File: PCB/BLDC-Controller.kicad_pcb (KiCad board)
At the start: 2 copper layers, 73 parts, among them Q1 Q_NMOS_GDS, Q2 Q_NMOS_GDS, Q3 Q_NMOS_GDS, Q4 Q_NMOS_GDS, Q5 Q_NMOS_GDS, Q6 Q_NMOS_GDS, U1 UCC27282DRM, U2 UCC27282DRM, U3 UCC27282DRM, U4 STM32F051K6Ux, U5 INA180A3, U6 TPS62933, Y1 8M

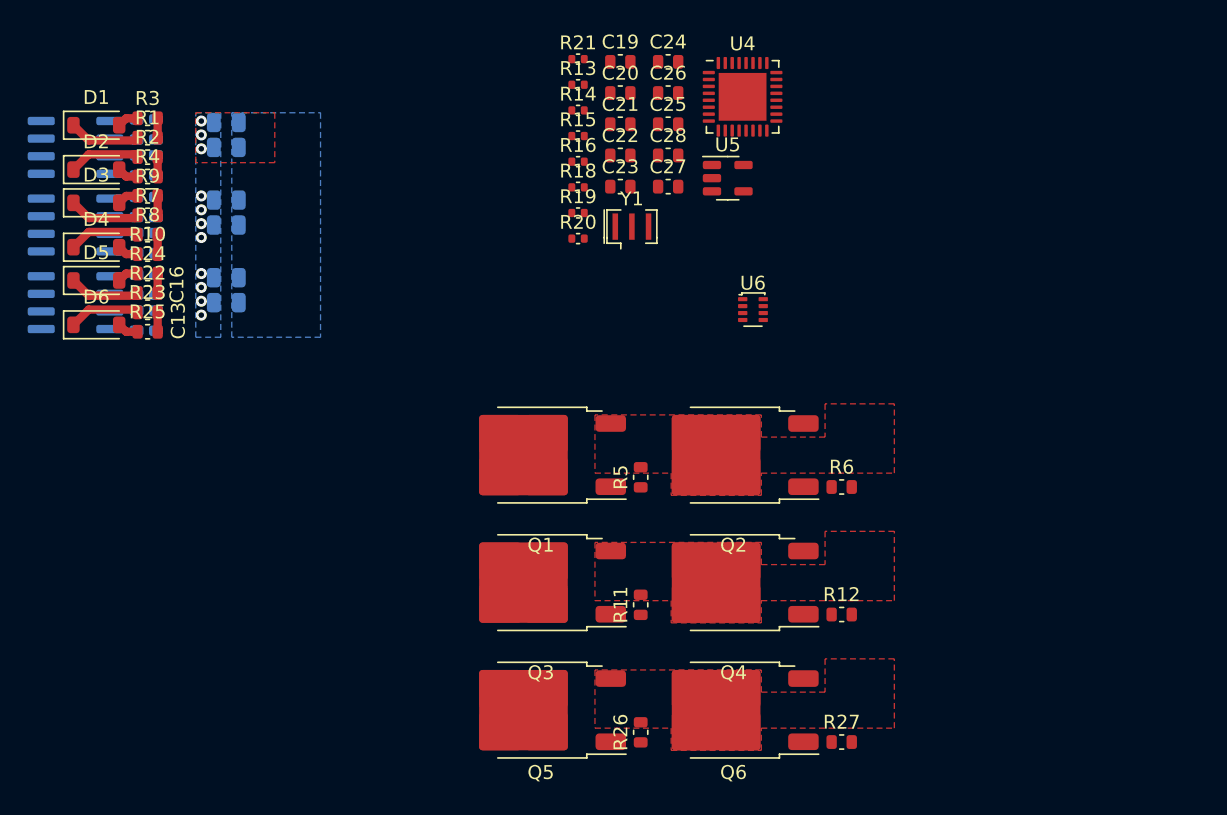
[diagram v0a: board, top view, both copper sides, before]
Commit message: f
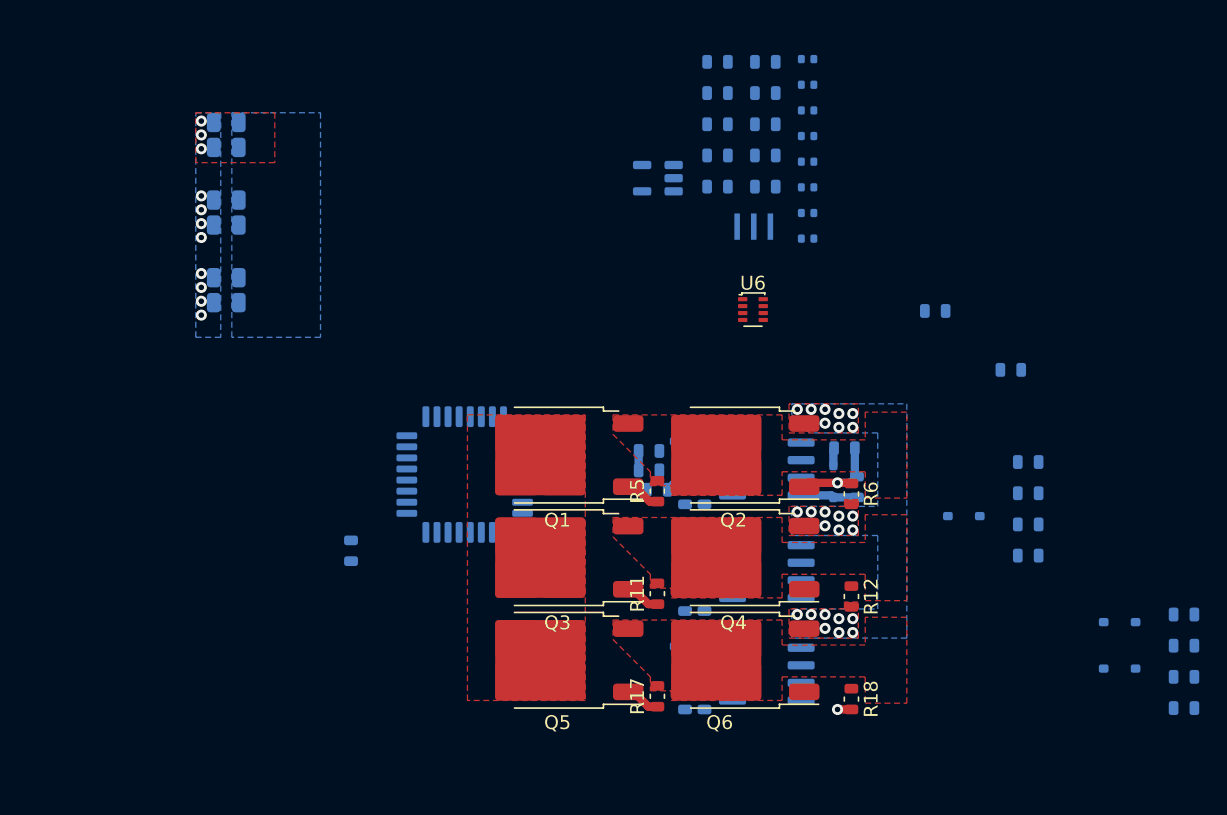
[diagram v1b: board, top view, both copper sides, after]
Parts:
- removed the C15 at (115.7, 95.4)
- removed the C3 at (115.7, 84.2)
- removed the C9 at (115.7, 89.8)
- removed the R22 at (116.5, 93.4)
- removed R23: 22, Ariamelon-Device:R_0603_1608Metric
- removed the R24 at (116.5, 92.0)
- removed the R25 at (116.5, 96.2)
- added L1: L_Small, Ariamelon-Device:L_0603_1608Metric, B.Cu at (153.3, 107.6)
- added L2: L_Small, Ariamelon-Device:L_0603_1608Metric, B.Cu at (178.8, 99.0)
- added L3: L_Small, Ariamelon-Device:L_0603_1608Metric, B.Cu at (173.3, 94.7)
- added R13: 10, Ariamelon-Device:R_0603_1608Metric, B.Cu at (180.1, 105.6)
- added R14: 10, Ariamelon-Device:R_0603_1608Metric, B.Cu at (180.1, 107.8)
- added R15: 22, Ariamelon-Device:R_0603_1608Metric, B.Cu at (180.1, 110.1)
- added R16: 22, Ariamelon-Device:R_0603_1608Metric, B.Cu at (180.1, 112.3)
- C16: renamed from C19; moved to B.Cu
- C17: renamed from C20; moved to B.Cu
- C18: renamed from C21; moved to B.Cu
- C19: renamed from C22; moved to B.Cu
- C20: renamed from C23; moved to B.Cu
- C21: renamed from C24; moved to B.Cu
- C22: renamed from C26; moved to B.Cu
- C23: renamed from C25; moved to B.Cu
- C24: renamed from C28; moved to B.Cu
- C25: renamed from C27; moved to B.Cu
- D1, D2, D3, D4, D5, D6: footprint Diode_SMD:D_SOD-123 -> Ariamelon-Device:D_SOD-323; moved to B.Cu
- Q1, Q2, Q3, Q4, Q5, Q6: footprint Package_TO_SOT_SMD:TO-252-2 -> Ariamelon-Package:TO-252-2
- R1, R2, R7, R8: value 22 -> 10; moved to B.Cu
- R10, R3, R4, R9: value 10 -> 22; moved to B.Cu
- R19: renamed from R21; moved to B.Cu
- R20: renamed from R13; moved to B.Cu
- R21: renamed from R14; moved to B.Cu
- R22: renamed from R15; moved to B.Cu
- R24: renamed from R16; moved to B.Cu
- R25: renamed from R18; moved to B.Cu
- R26: renamed from R19; moved to B.Cu
- R27: renamed from R20; moved to B.Cu
- U1, U2, U3: value UCC27282DRM -> UCC27211ADRM
- U4: value STM32F051K6Ux -> STM32F051K6Tx; footprint Package_DFN_QFN:QFN-32-1EP_5x5mm_P0.5mm_EP3.45x3.45mm -> Package_QFP:LQFP-32_7x7mm_P0.8mm; moved to B.Cu
- U5, Y1: moved to B.Cu
- moved R9 82.4 mm to (191.3, 121.1), turned to 180 degrees
- moved R10 81.6 mm to (191.3, 123.3), turned to 180 degrees
- moved R8 80.4 mm to (191.3, 118.8), turned to 180 degrees
- moved R7 80.1 mm to (191.3, 116.6), turned to 180 degrees
- moved D4 79.8 mm to (186.7, 120.5), turned to 180 degrees
- moved D3 79.8 mm to (186.7, 117.2), turned to 180 degrees
- moved D6 64.1 mm to (175.4, 109.5), turned to 180 degrees
- moved D2 57.7 mm to (166.0, 107.0), turned to 90 degrees
- moved U3 56.6 mm to (161.2, 120.9), turned to 0 degrees
- moved R4 55.9 mm to (167.7, 107.4), turned to 90 degrees
- moved U2 55.8 mm to (161.2, 113.5), turned to 0 degrees
- moved U1 55.0 mm to (161.2, 106.1), turned to 0 degrees
- moved R2 54.5 mm to (166.8, 104.6)
- moved C12 50.7 mm to (156.7, 122.7)
- moved D5 50.4 mm to (155.7, 118.9), turned to 180 degrees
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- renumbered C12 to C10, C13 to C11, C14 to C12, C16 to C13, C17 to C14, C18 to C15, C4 to C3, C5 to C4, C6 to C5, C7 to C6, C8 to C7, C10 to C8, C11 to C9, R26 to R17, R27 to R18
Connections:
- R1 pad 1: Net-(D1-K) -> Net-(D1-A)
- R10 pad 1: Net-(D4-A) -> Net-(D4-K)
- R2 pad 1: Net-(D2-K) -> Net-(D2-A)
- R3 pad 1: Net-(D1-A) -> Net-(D1-K)
- R4 pad 1: Net-(D2-A) -> Net-(D2-K)
- R7 pad 1: Net-(D3-K) -> Net-(D3-A)
- R8 pad 1: Net-(D4-K) -> Net-(D4-A)
- R9 pad 1: Net-(D3-A) -> Net-(D3-K)
- U4 pad 13: /MCU/LI_C -> /MCU/LI_A
- U4 pad 15: /MCU/LI_A -> /MCU/LI_C
- U4 pad 16: unconnected-(U4-PB2-Pad16) -> GND
- U4 pad 18: /MCU/HI_C -> /MCU/HI_A
- U4 pad 20: /MCU/HI_A -> /MCU/HI_C
- U4 pad 32: unconnected-(U4-PB8-Pad32) -> GND
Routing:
- net Net-(Q2-G): track 1.40 -> 6.95 mm, vias 0 -> 1
- net Net-(D6-K): track 5.16 -> 0.00 mm
- net Net-(D1-K): track 5.16 -> 0.00 mm
- net Net-(D4-K): track 5.16 -> 0.00 mm
- net Net-(D3-K): track 5.16 -> 0.00 mm
- net Net-(D5-K): track 5.16 -> 0.00 mm
- net Net-(U1-VDD): track 0.00 -> 2.84 mm
- net Net-(Q1-G): track 1.40 -> 3.46 mm
- net Net-(D6-A): track 1.53 -> 0.00 mm
- net Net-(D5-A): track 1.53 -> 0.00 mm
- net Net-(D4-A): track 1.53 -> 0.00 mm
- net Net-(D3-A): track 1.53 -> 0.00 mm
- net Net-(D1-A): track 1.53 -> 0.00 mm
- net Net-(Q6-G): track 1.40 -> 0.00 mm
- net Net-(Q4-G): track 1.40 -> 0.00 mm
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- added copper zone on F.Cu, net VCC
